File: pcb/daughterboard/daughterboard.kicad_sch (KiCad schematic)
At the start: 2 parts, among them J1 Conn_01x05_Pin, J22 Conn_01x05_Pin

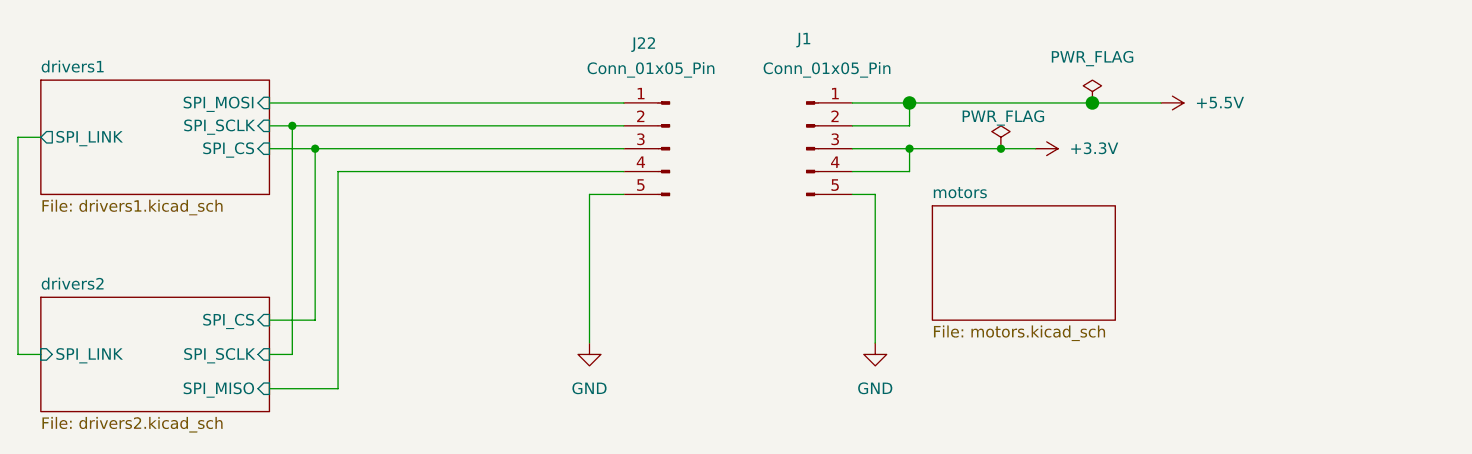
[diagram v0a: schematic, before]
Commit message: added initial power lines
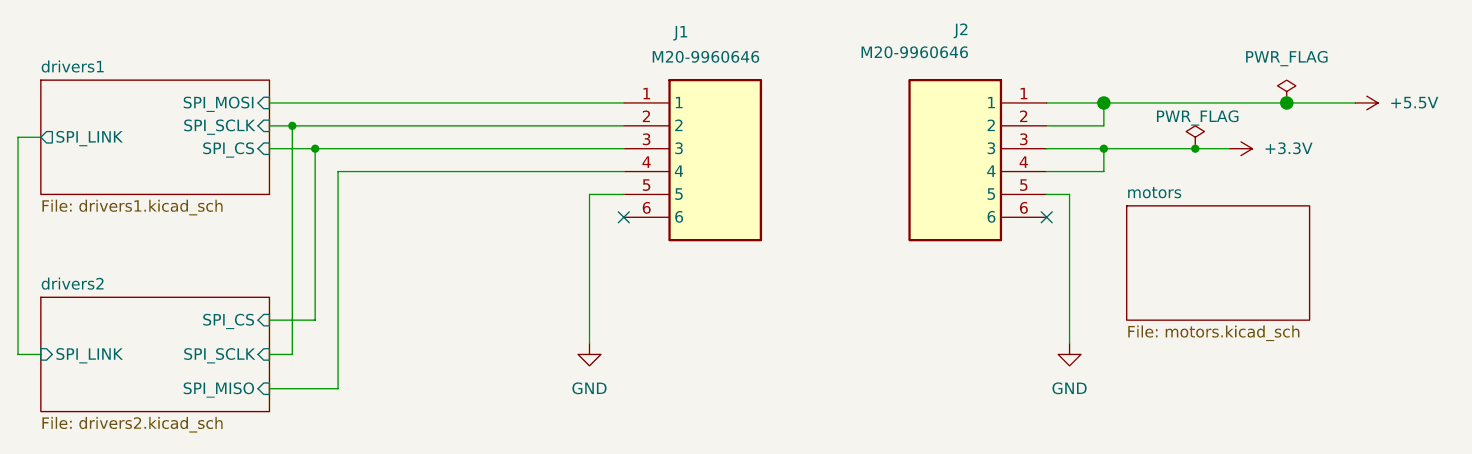
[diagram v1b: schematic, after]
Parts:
- removed J1, J22: Conn_01x05_Pin, symbol Connector:Conn_01x05_Pin
- added J1, J2: M20-9960646, A_HANU_FOOTPRINTS:HDRRA6W64P0X254_1X6_1524X254X254P, symbol M20-9960646:M20-9960646
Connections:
- net +3.3V: now also J2.3, J2.4
- net +5.5V: now also J2.1, J2.2
- net GND: now also J1.5, J2.5
- net drivers1/SPI_CS: now also J1.3
- net drivers1/SPI_MOSI: now also J1.1
- net drivers1/SPI_SCLK: now also J1.2
- net drivers2/SPI_MISO: now also J1.4
- no-connect marks 0 -> 2
